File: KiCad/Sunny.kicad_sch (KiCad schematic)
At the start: 11 parts, among them J1 VIN (7V5-40VDC), J2 GND, J5 USB_A

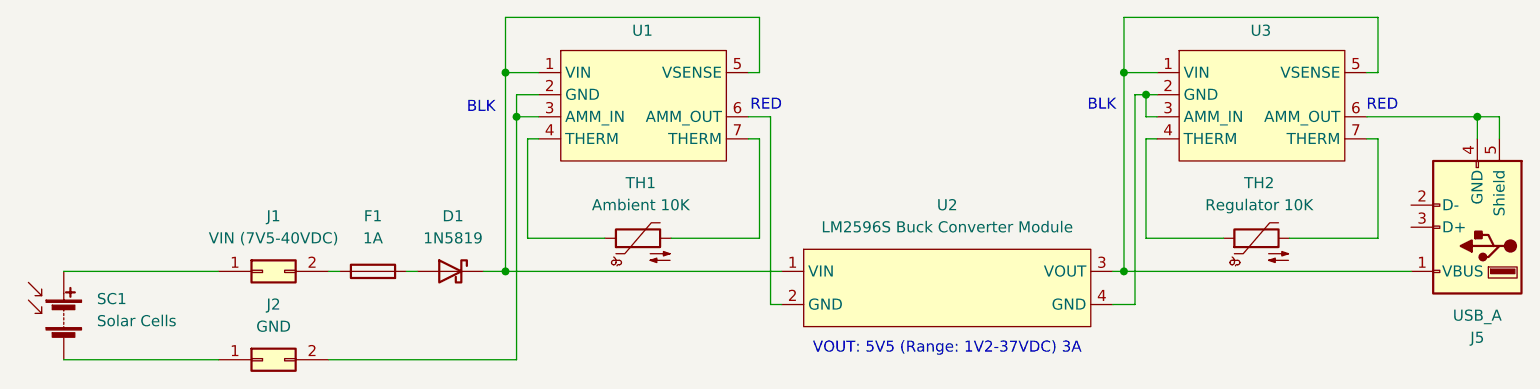
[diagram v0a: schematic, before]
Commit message: Review
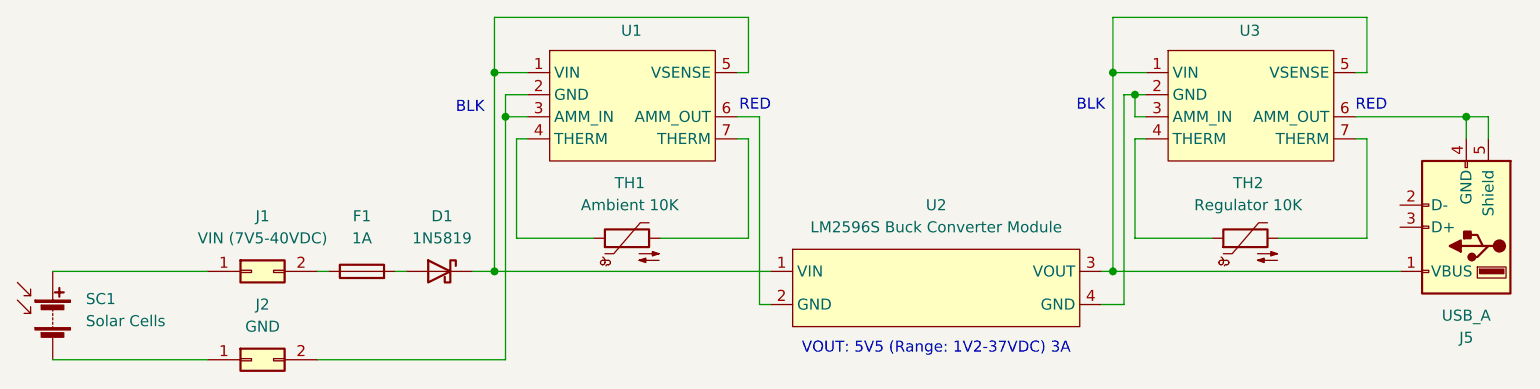
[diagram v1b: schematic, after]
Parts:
- U1, U2, U3: value ~ -> (none)
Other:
- moved on the sheet: D1, F1, J1, J2, J5, SC1, TH1, TH2, U1, U2, U3
